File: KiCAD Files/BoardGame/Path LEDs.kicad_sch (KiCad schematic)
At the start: 53 parts

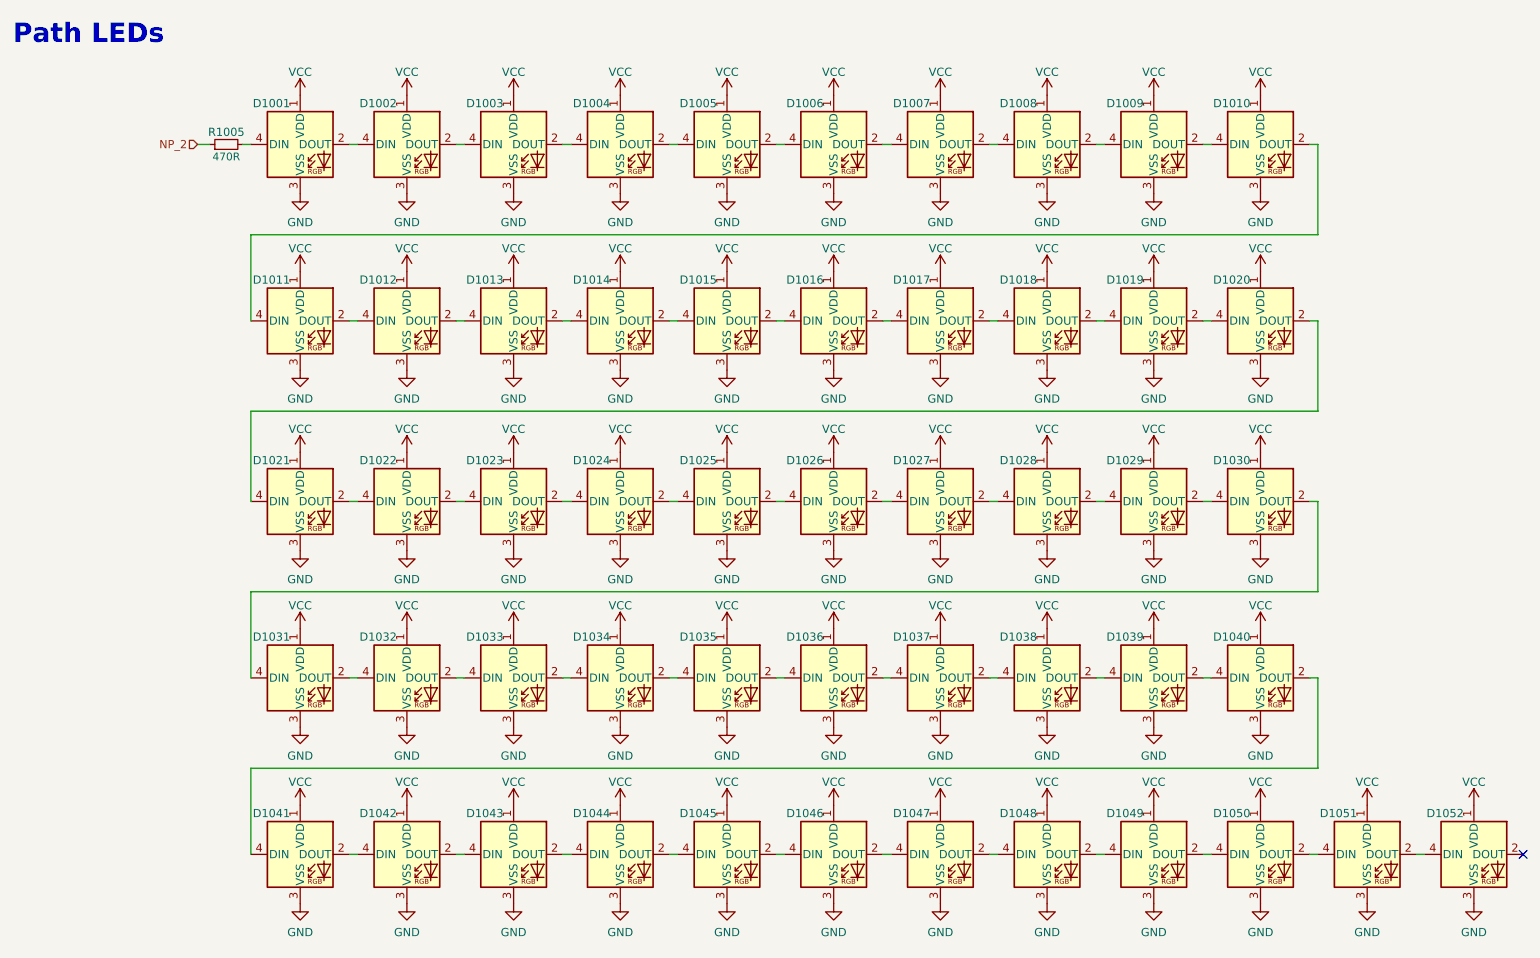
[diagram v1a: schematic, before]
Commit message: update
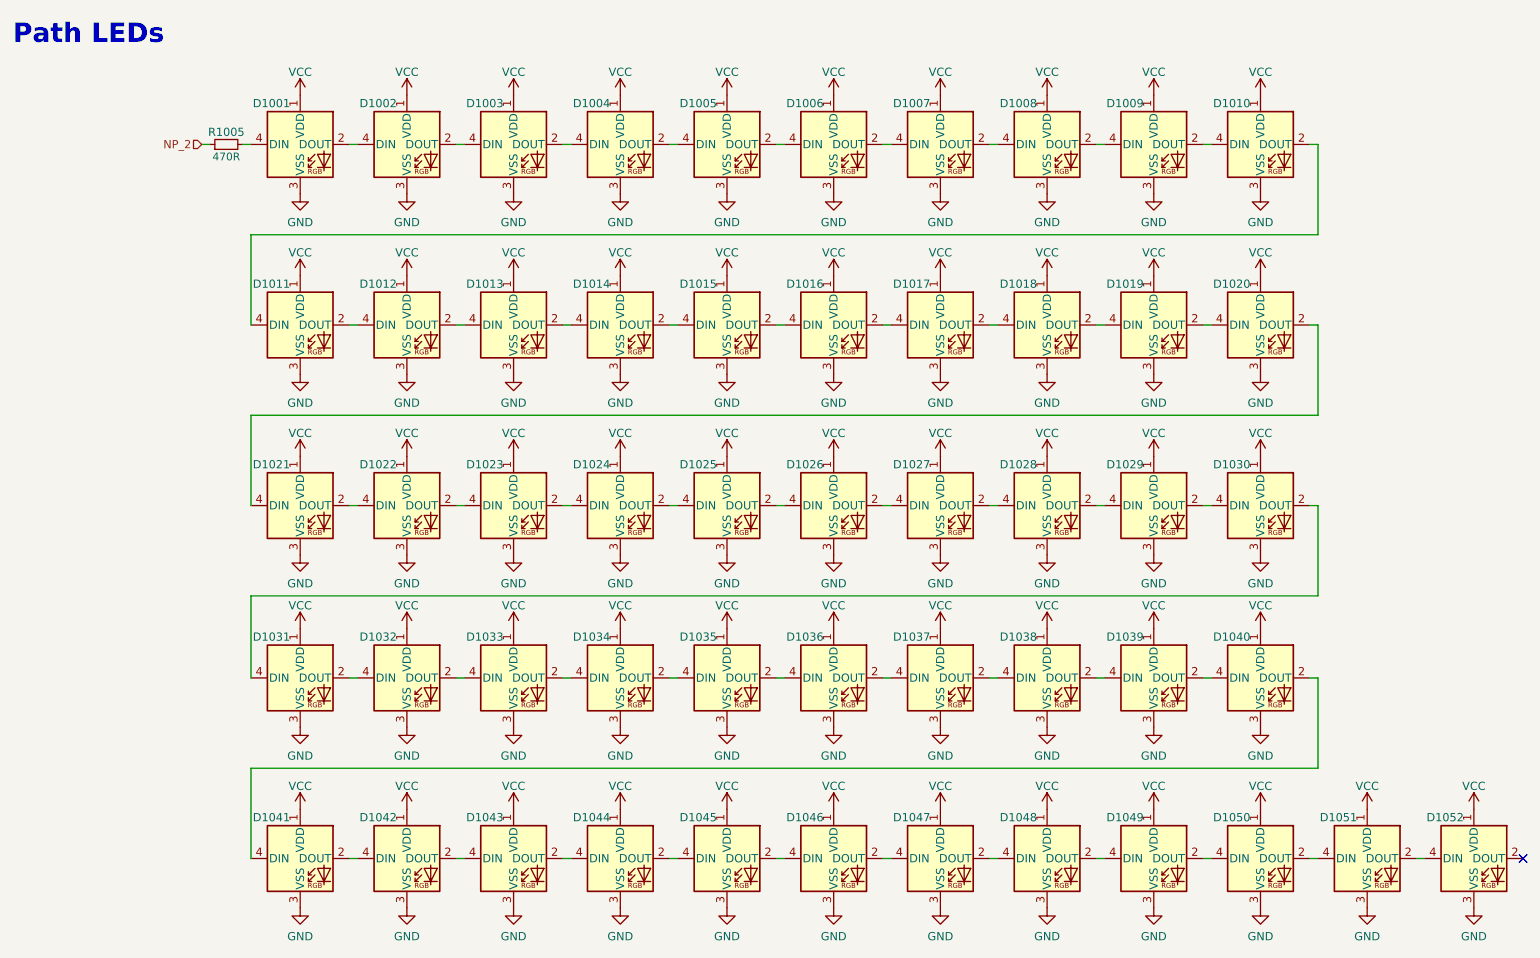
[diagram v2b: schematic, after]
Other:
- moved on the sheet: D1011, D1012, D1013, D1014, D1015, D1016, D1017, D1018, D1019, D1020, D1021, D1022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
